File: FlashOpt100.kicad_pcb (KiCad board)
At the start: 2 copper layers, 16 x 38 mm, 8 parts, among them J1 Tandy_100_102_200_option_rom, J2 FlashOpt100_PRG_4x7, U1 29F010 TSOP

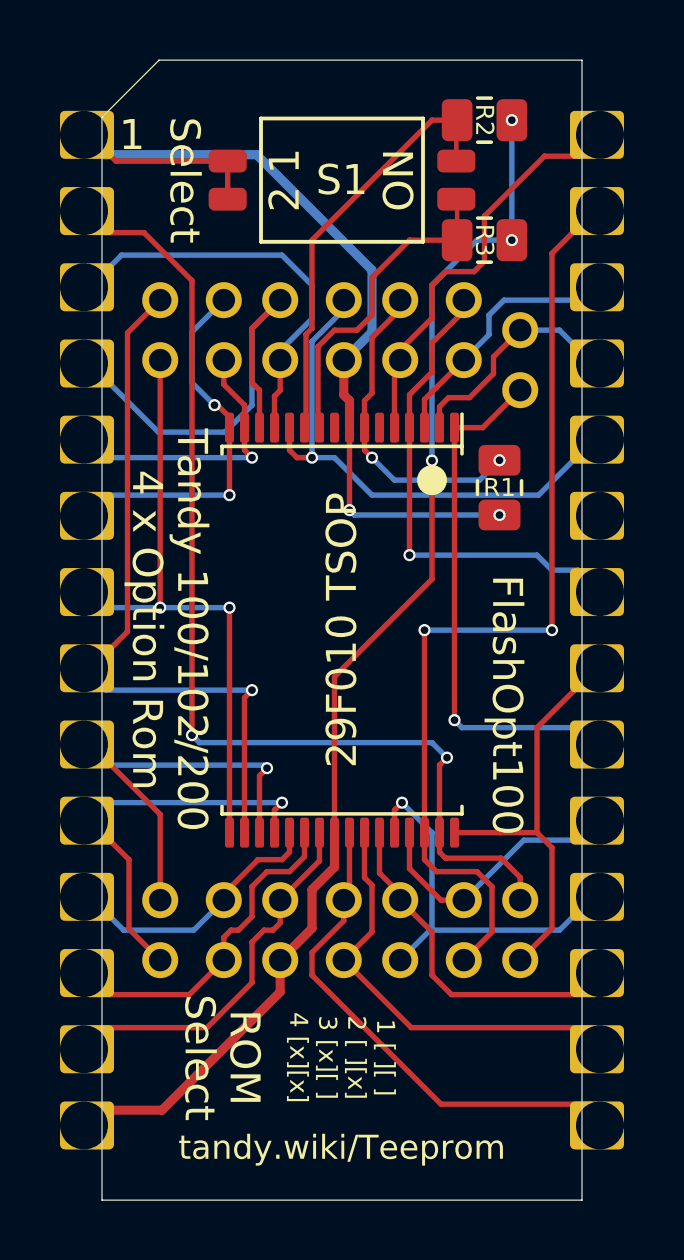
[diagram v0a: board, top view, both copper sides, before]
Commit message: cosmetics
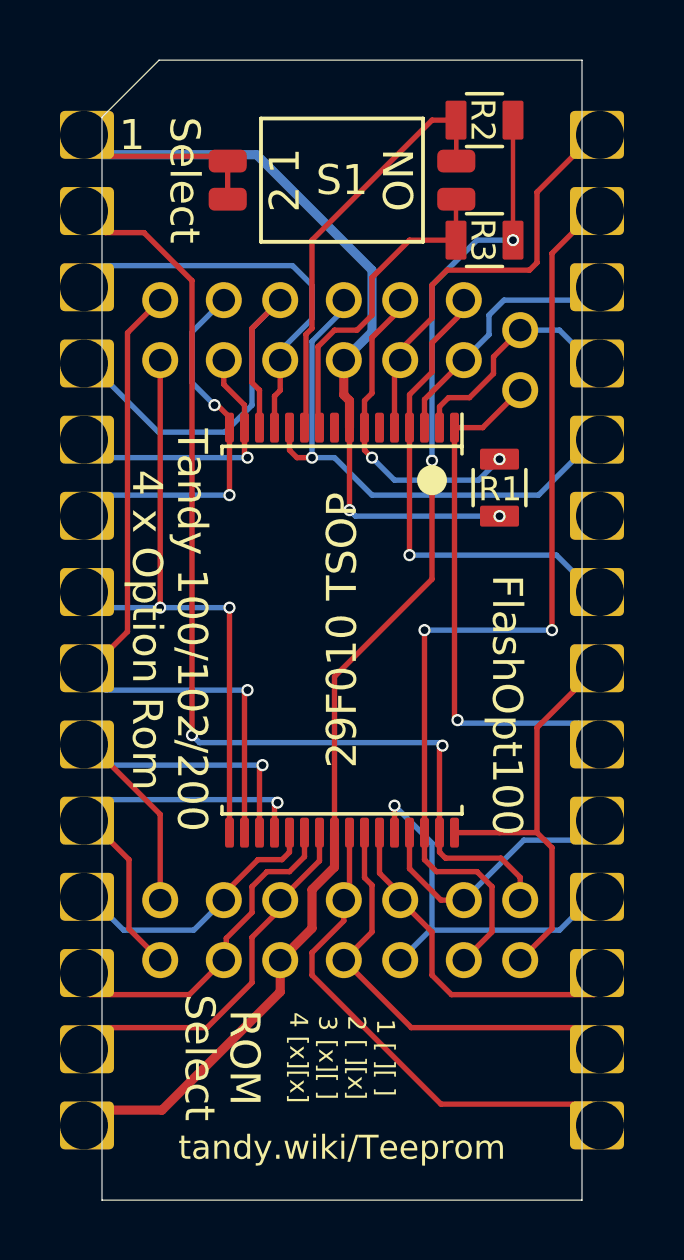
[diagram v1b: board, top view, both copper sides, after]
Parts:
- R1, R2, R3: footprint 000_LOCAL:R_0805_2012Metric -> 000_LOCAL:R_0805
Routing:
- net GND: track 41.3 -> 41.4 mm, vias 3 -> 2

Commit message: update to v004 board outline and carrier
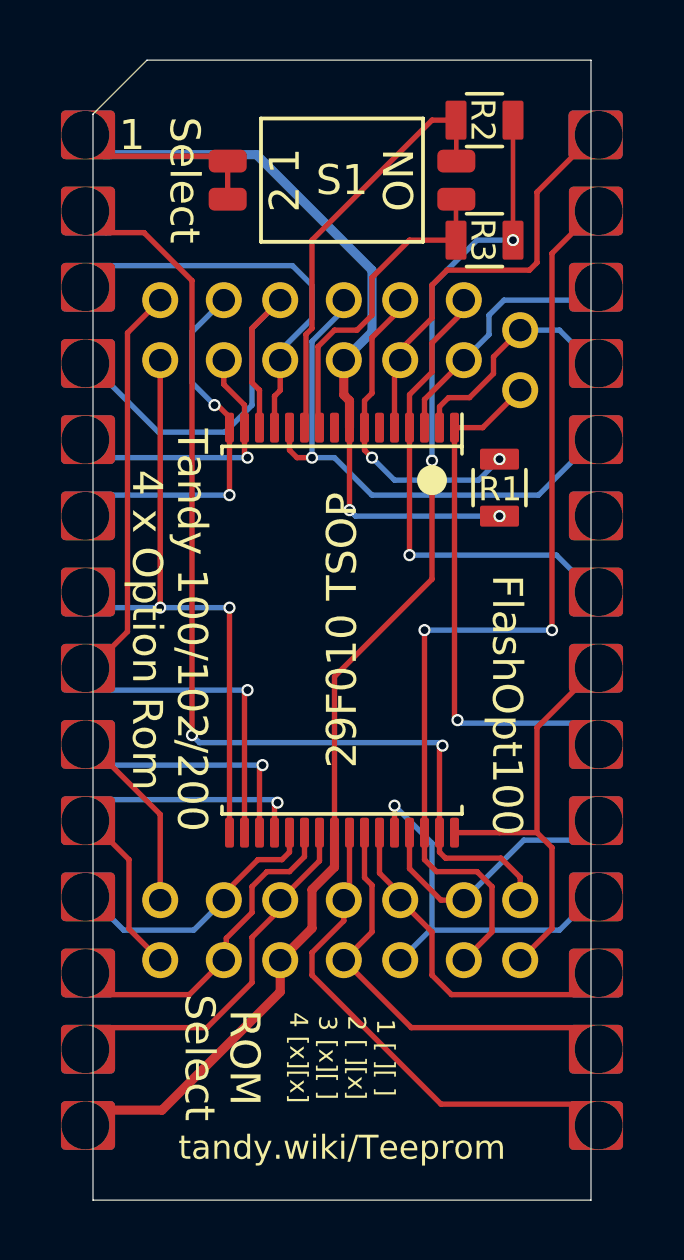
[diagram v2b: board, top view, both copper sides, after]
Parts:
- removed carrier?: pcb2molex8878_chamfer, 000_LOCAL:pcb2molex8878_chamfer
- J1: footprint 000_LOCAL:pcb2molex8878 -> 000_LOCAL:Molex78802_PCB_28
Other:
- board size 16 x 38 mm -> 16.6 x 38 mm
- board text added: "v004"
